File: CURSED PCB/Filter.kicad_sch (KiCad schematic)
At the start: 4 parts, among them U10 OPA2314AIDR, U9 OPA2314AIDR

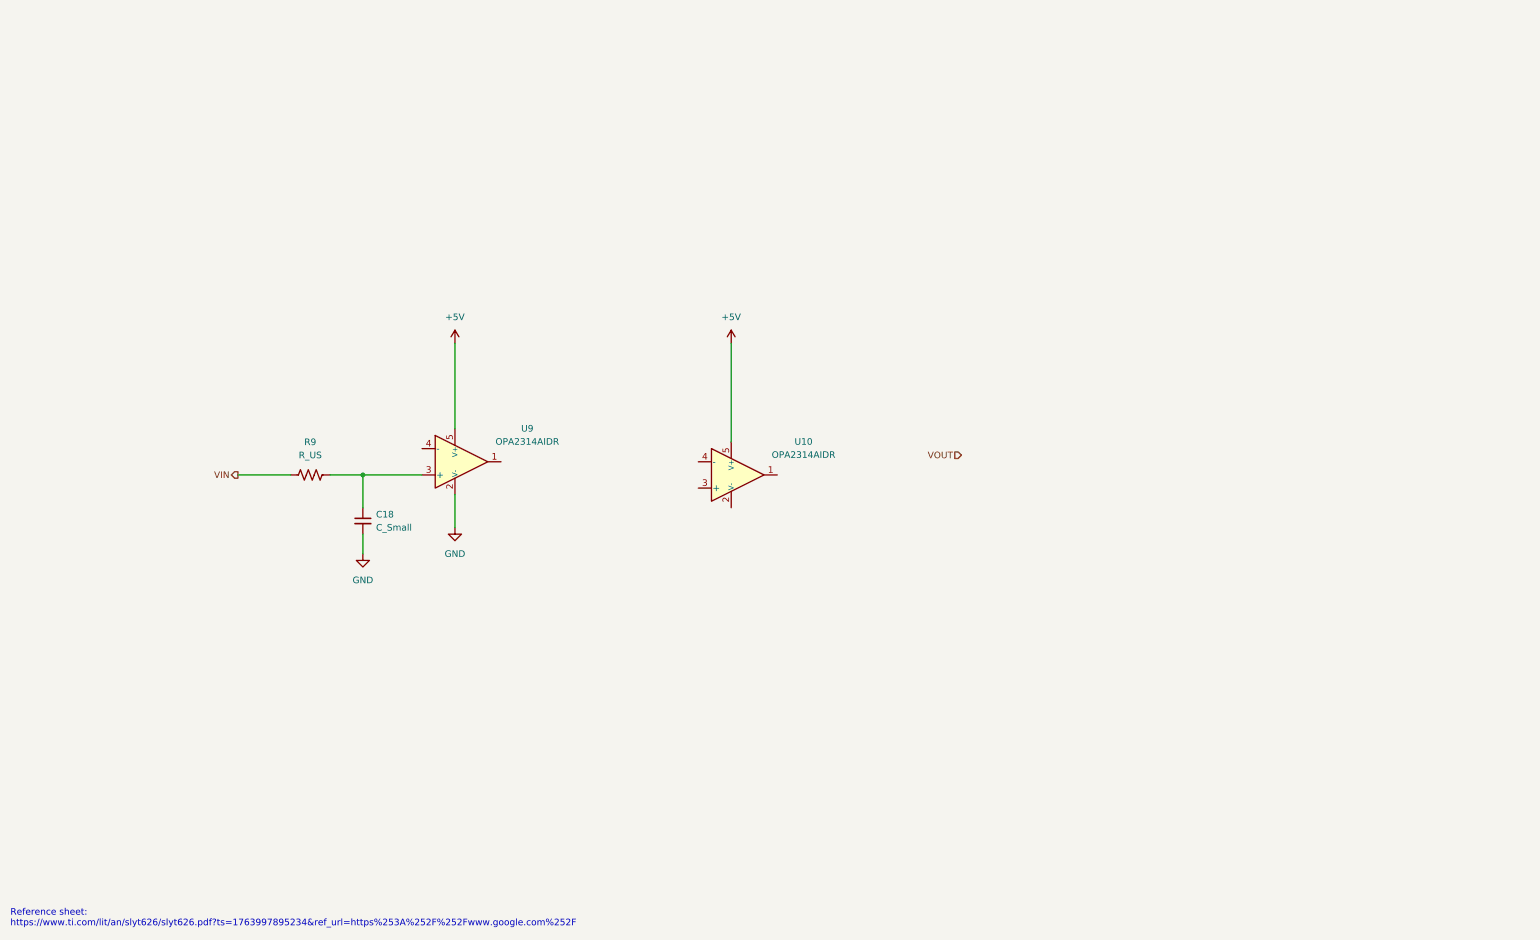
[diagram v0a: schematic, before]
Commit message: Updates to PCB before exam sesaon
idk what I added ngl
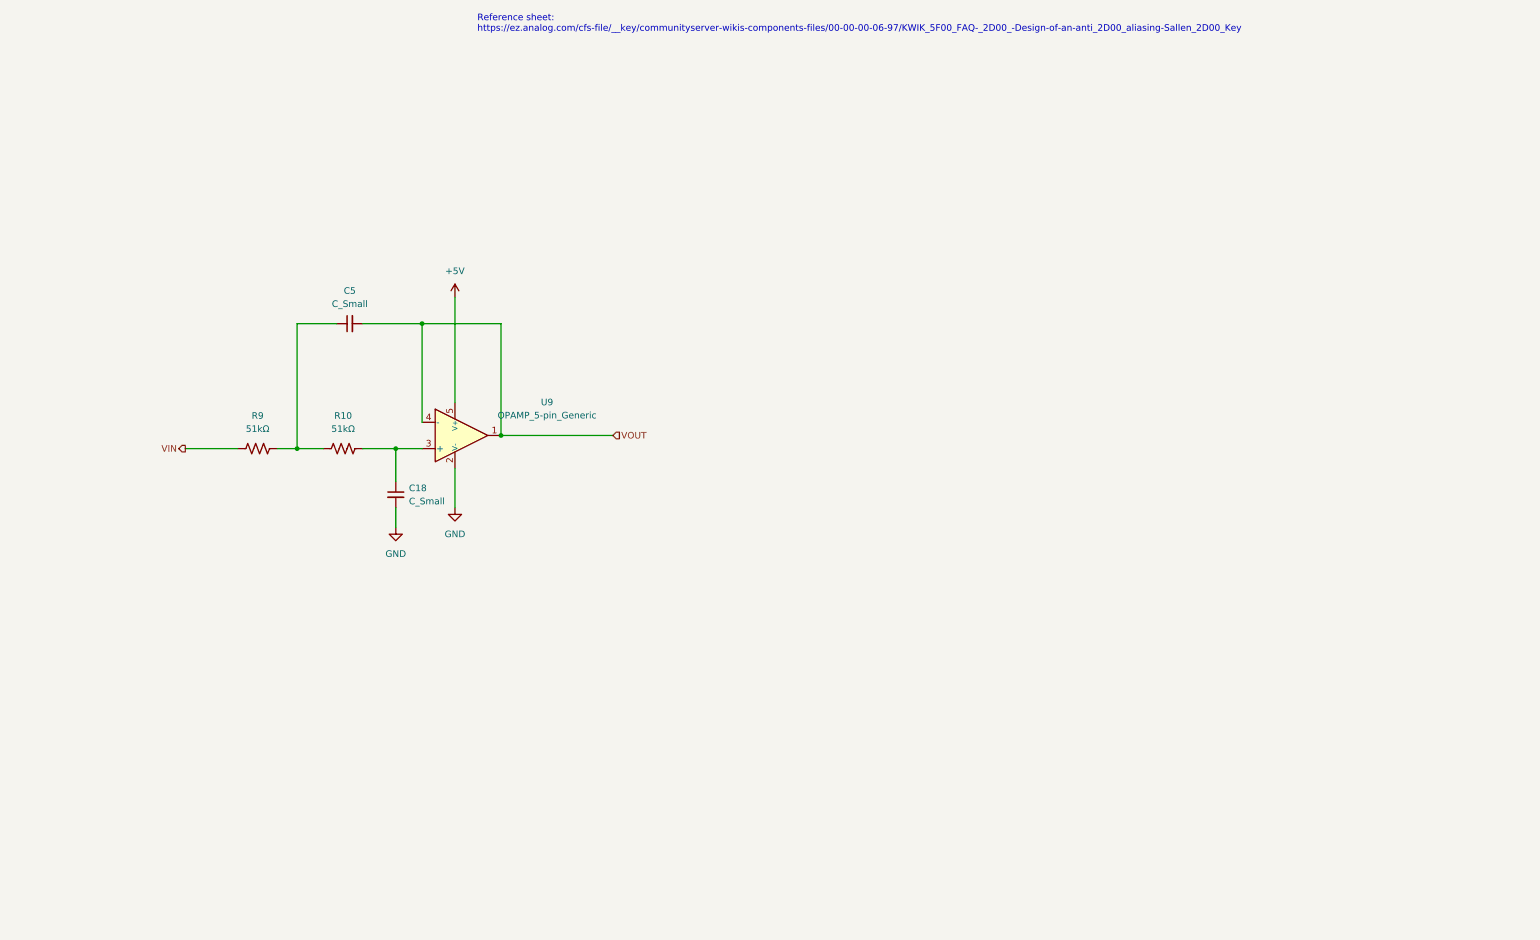
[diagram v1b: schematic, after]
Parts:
- removed U10, U9: OPA2314AIDR, PCM_Package_TO_SOT_SMD_AKL:SOT-23-5, symbol PCM_Amplifier_Operational_AKL:OPA313IDBV
- added C5: C_Small, symbol Device:C_Small
- added R10: 51kΩ, symbol Device:R_US
- added U9: OPAMP_5-pin_Generic, Package_TO_SOT_SMD:SOT-23-5, symbol PCM_Amplifier_Operational_AKL:OPAMP_5-pin_Generic
- R9: value R_US -> 51kΩ
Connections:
- net +5V: now also U9.5 (V+)
- net GND: now also U9.2 (V-)
- net VOUT: now also C5.2, U9.1, U9.4 (-)
- net at R9.2: now also C5.1, R10.1; no longer C18.1
- new net: C18.1, R10.2, U9.3 (+)
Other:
- note added: "Reference sheet: https://ez.analog.com/cfs-file/__key/communityserver-wikis-components-files/00-00-00-06-97/KWIK_5F00_FAQ-_2D00_-Design-of-an-anti_2D00_aliasing-Sallen_2D00_Key"
- note removed: "Reference sheet: https://www.ti.com/lit/an/slyt626/slyt626.pdf?ts=1763997895234&ref_url=https%253A%252F%252Fwww.google.com%252F"
- moved on the sheet: C18, R9
